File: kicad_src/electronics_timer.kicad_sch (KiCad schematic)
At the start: 21 parts, among them U1 CD4013BE

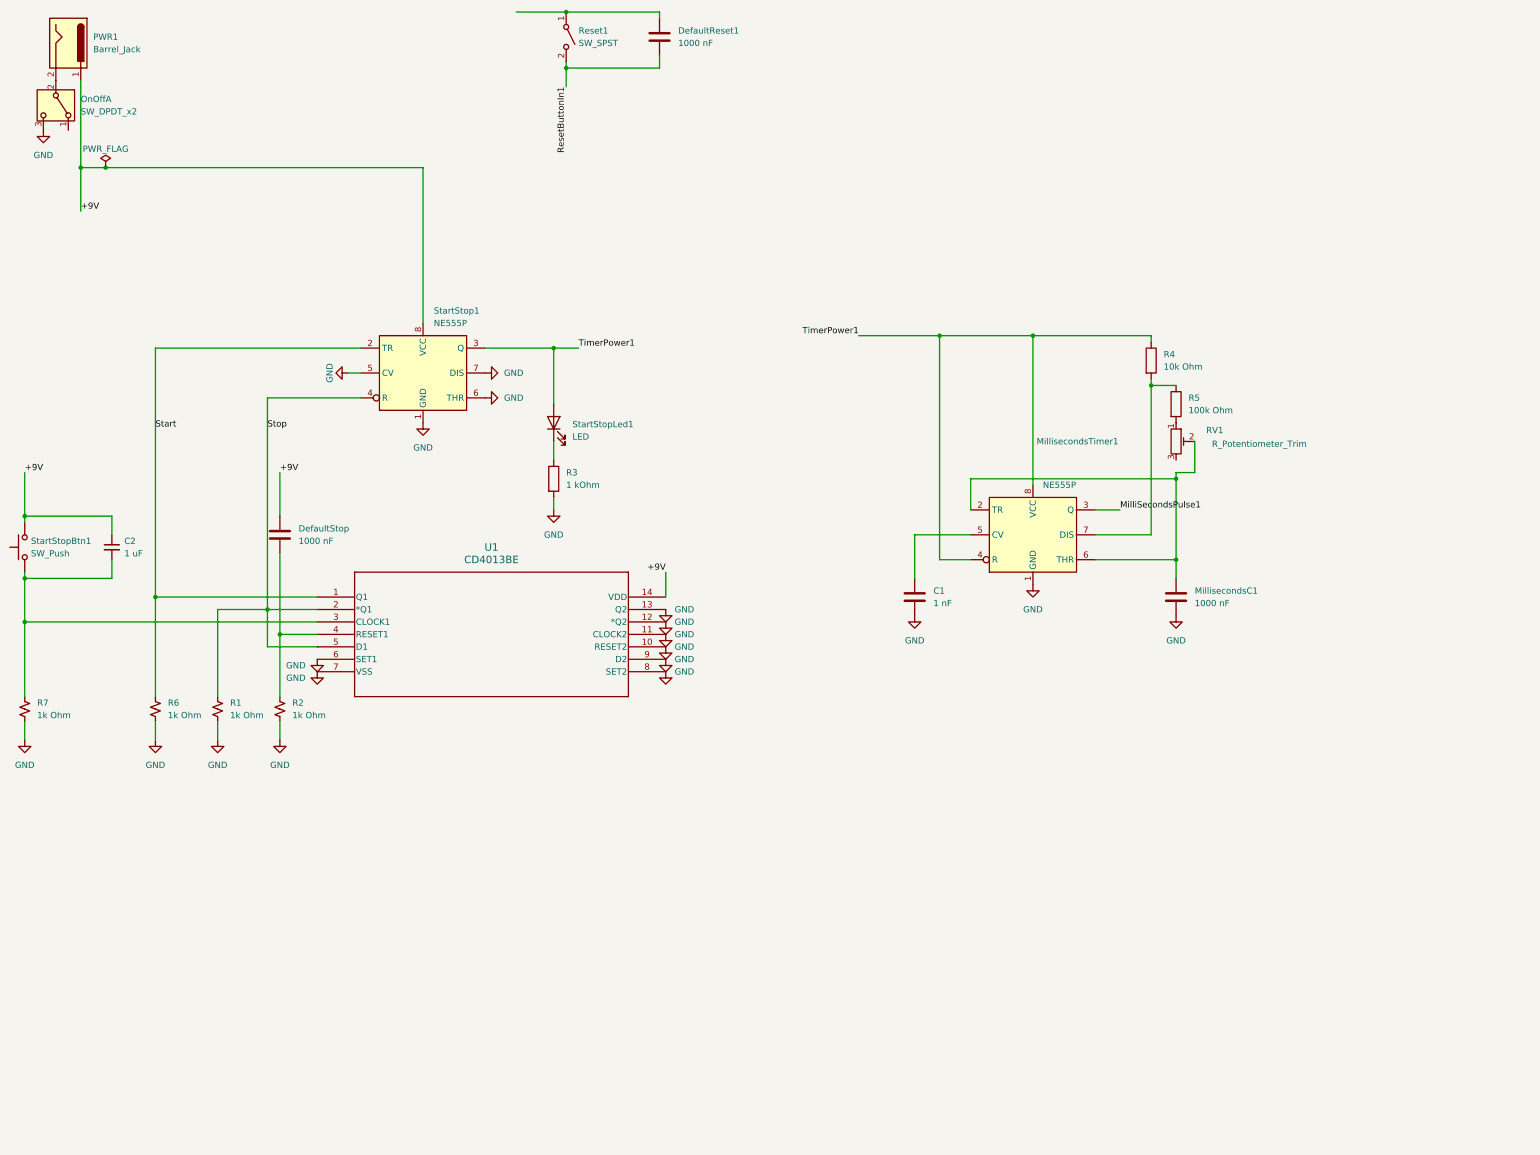
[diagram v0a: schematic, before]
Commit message: save progress, set up down in simple way done
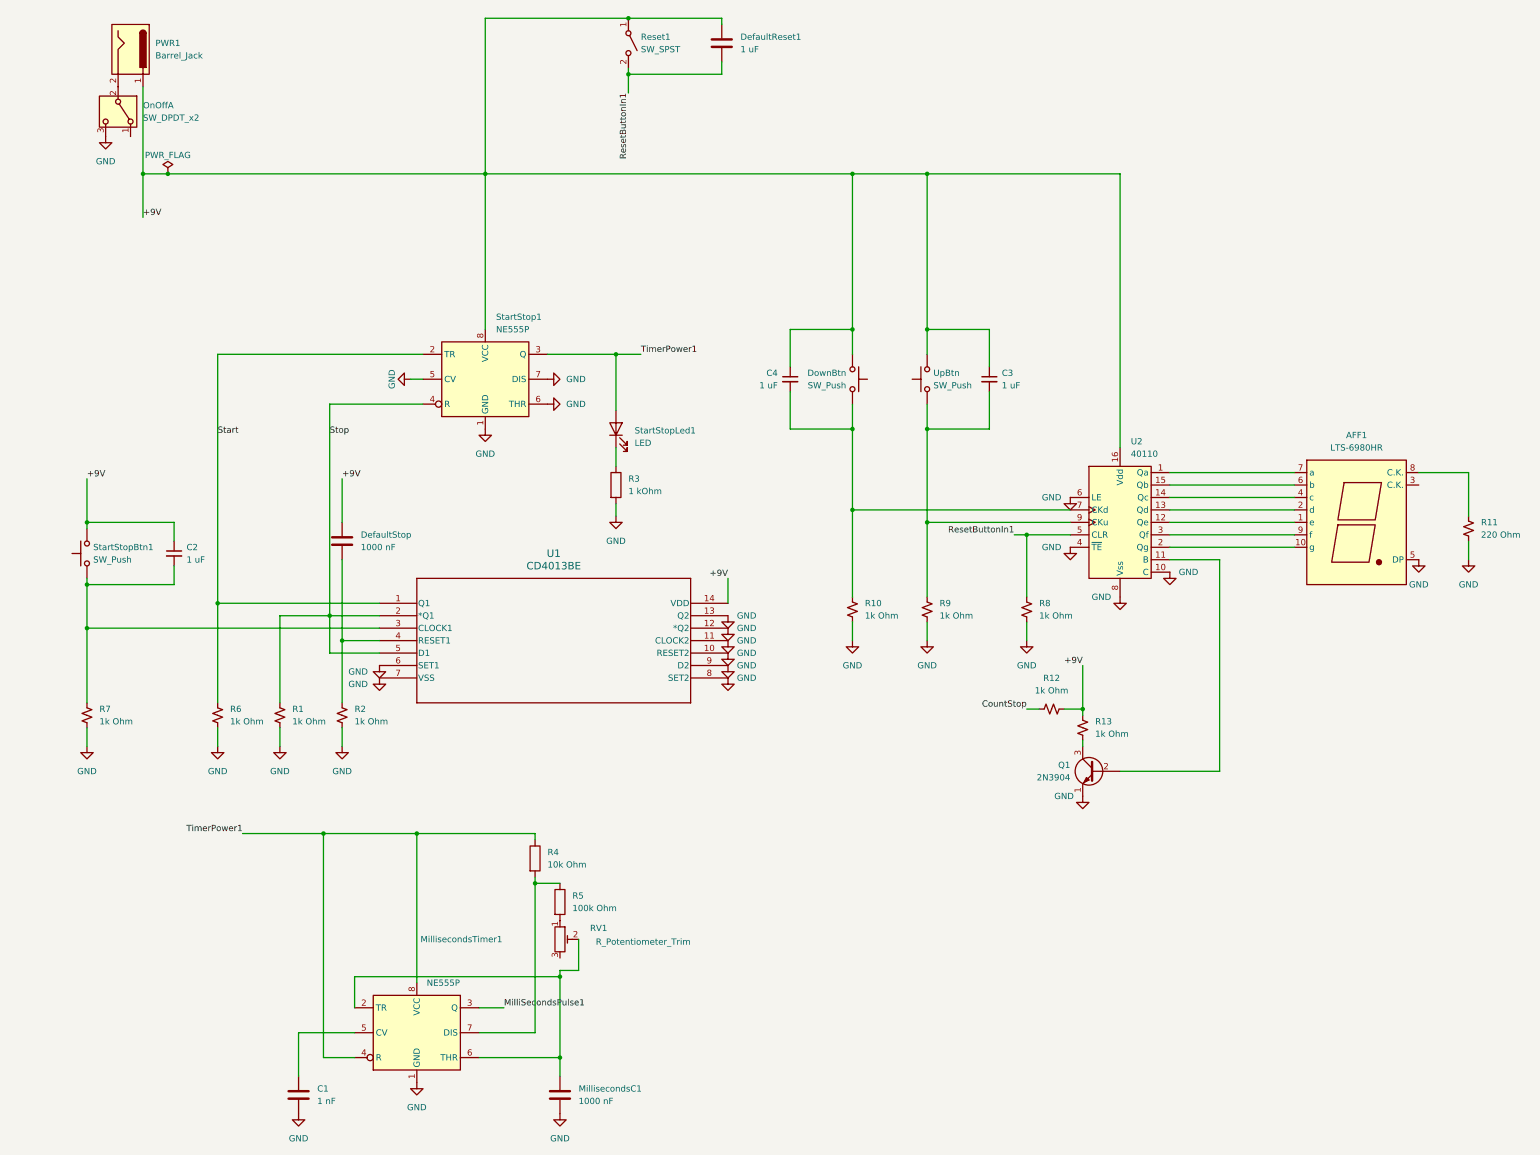
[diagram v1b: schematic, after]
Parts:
- added AFF1: LTS-6980HR, Display_7Segment:7SegmentLED_LTS6760_LTS6780, symbol Display_Character:LTS-6980HR
- added C3, C4: 1 uF, symbol Device:C_Small
- added DownBtn, UpBtn: SW_Push, symbol Switch:SW_Push
- added Q1: 2N3904, Package_TO_SOT_THT:TO-92_Inline, symbol Transistor_BJT:2N3904
- added R10, R12, R13, R8, R9: 1k Ohm, symbol Device:R_Small_US
- added R11: 220 Ohm, symbol Device:R_Small_US
- added U2: 40110, symbol 4xxx_IEEE:40110
- DefaultReset1: value 1000 nF -> 1 uF
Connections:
- net +9V: now also DefaultReset1.1, Reset1.1 (A), C3.1, C4.1, DownBtn.2, R12.1, R13.2, U2.16 (Vdd), UpBtn.2
- net GND: now also AFF1.5 (DP), Q1.1 (E), R10.2, R11.2, R8.2, R9.2, U2.10 (C), U2.4 (~{TE}), U2.6 (LE), U2.8 (Vss)
- net ResetButtonIn1: now also R8.1, U2.5 (CLR)
- new net: C4.2, DownBtn.1, R10.1, U2.7 (CKd)
- new net: C3.2, R9.1, U2.9 (CKu), UpBtn.1
- new net: Q1.3 (C), R13.1
- new net: AFF1.1 (e), U2.12 (Qe)
- new net: AFF1.10 (g), U2.2 (Qg)
- new net: AFF1.2 (d), U2.13 (Qd)
- new net: AFF1.4 (c), U2.14 (Qc)
- new net: AFF1.6 (b), U2.15 (Qb)
- new net: AFF1.7 (a), U2.1 (Qa)
- new net: AFF1.8 (C.K.), R11.1
- new net: AFF1.9 (f), U2.3 (Qf)
- new net: Q1.2 (B), U2.11 (B)
- new net CountStop: R12.2
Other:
- moved on the sheet: C1, C2, DefaultReset1, DefaultStop, MillisecondsC1, MillisecondsTimer1, OnOffA, PWR1, R1, R2, R3, R4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
